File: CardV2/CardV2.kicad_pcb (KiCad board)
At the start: 2 copper layers, 40 x 40 mm, 4 parts, among them U1 M24LR04E-R

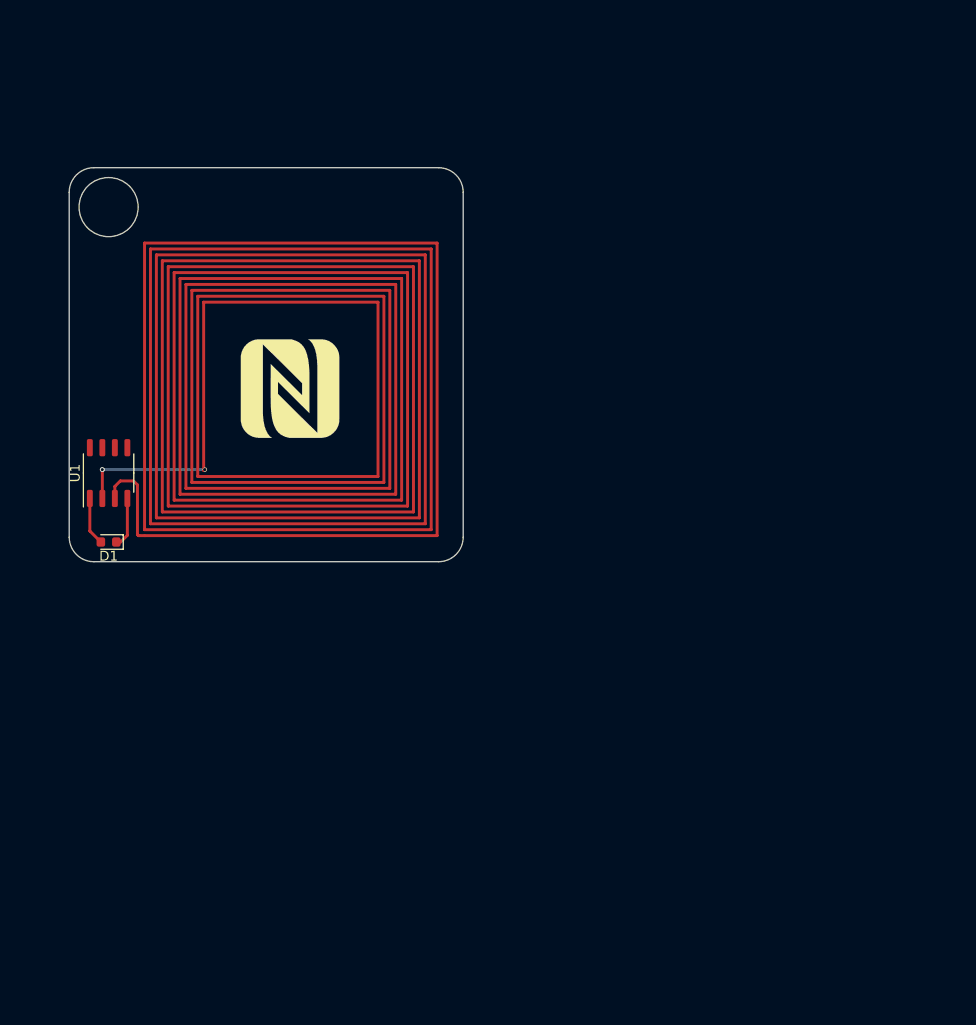
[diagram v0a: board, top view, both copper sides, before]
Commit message: 失败的拼版
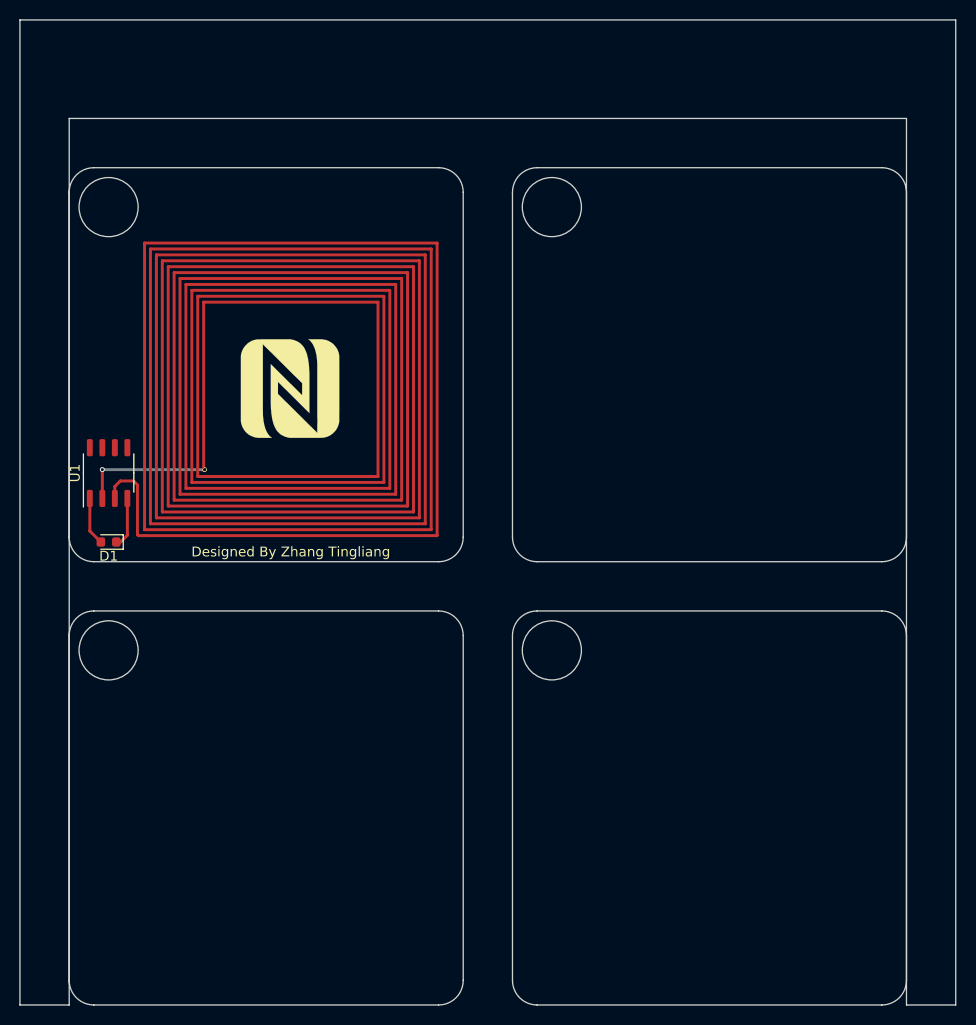
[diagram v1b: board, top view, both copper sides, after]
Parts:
- added G***: LOGO, CardV2:FutureLabLogo, B.Cu at (122.5, 82.5)
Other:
- board size 40 x 40 mm -> 95 x 100 mm
- board text added: "Designed By Zhang Tingliang"
